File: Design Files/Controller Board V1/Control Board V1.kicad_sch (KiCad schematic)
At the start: 7 parts, among them IC1 LMR66410MC5RXBRQ1

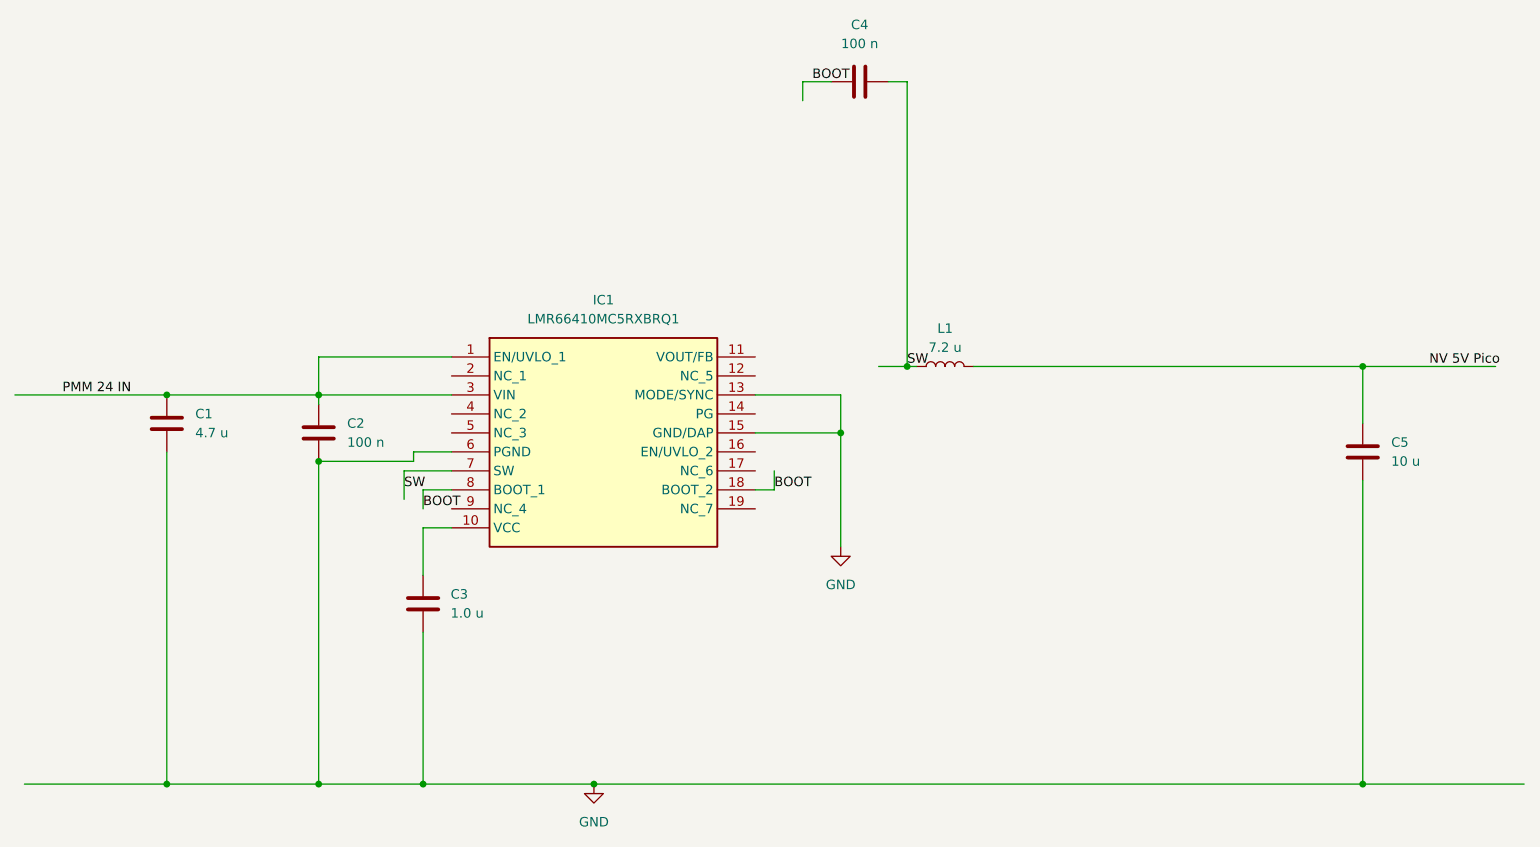
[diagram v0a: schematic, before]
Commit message: 5v
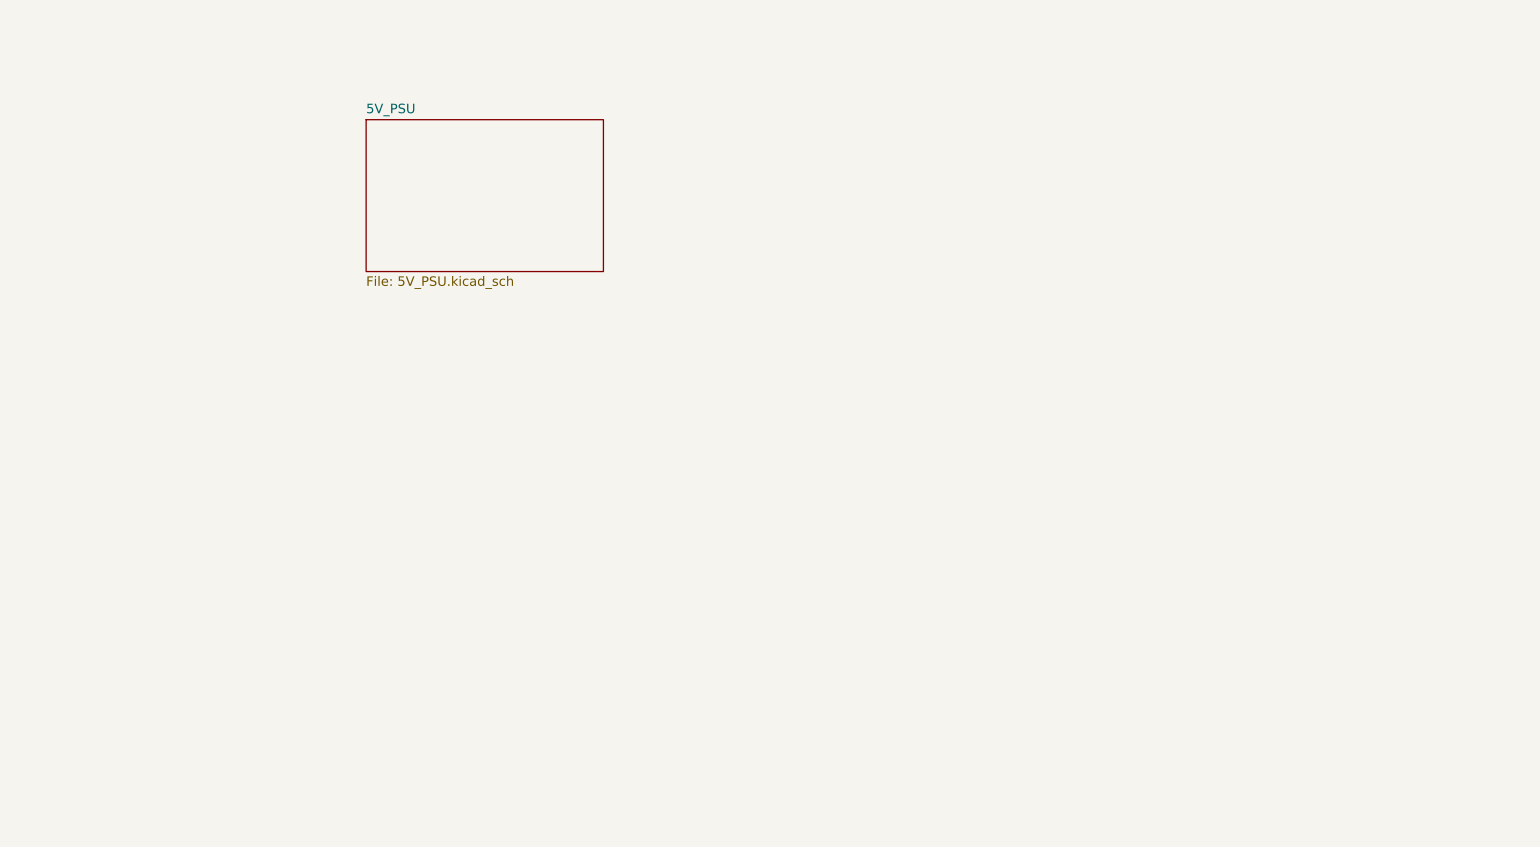
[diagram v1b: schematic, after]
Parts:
- removed C1: 4.7 u, symbol Device:C
- removed C2, C4: 100 n, symbol Device:C
- removed C3: 1.0 u, symbol Device:C
- removed C5: 10 u, symbol Device:C
- removed IC1: LMR66410MC5RXBRQ1, LMR66430R5RXBR, symbol LMR66410MC5RXBRQ1:LMR66410MC5RXBRQ1
- removed L1: 7.2 u, symbol Device:L
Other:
- added sheet 5V_PSU (5V_PSU.kicad_sch)
